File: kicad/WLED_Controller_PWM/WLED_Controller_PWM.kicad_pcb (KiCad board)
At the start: 2 copper layers, 72 x 50 mm, 45 parts, among them J1 USB_C_Receptacle_USB2.0, J2 Conn_01x03, J3 Conn_01x03, J4 Conn_01x03, J6 Conn_01x02, Q1 BC847, Q2 BC847, SW1 SW_RESET, SW2 SW_BOOT, SW3 SW_Push, U1 ESP32-WROOM-32, U2 CH340C, U3 NCP1117-3.3, U4 TSSP58P38, U5 74HC14

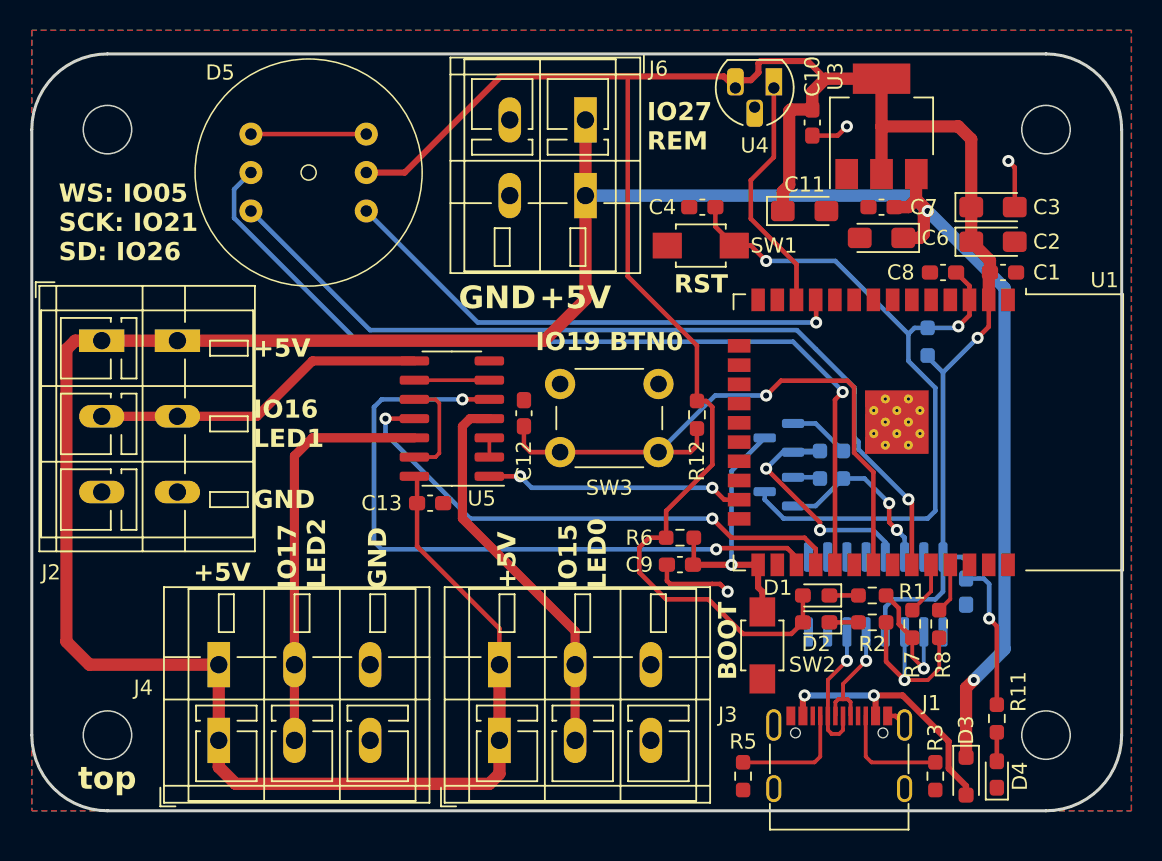
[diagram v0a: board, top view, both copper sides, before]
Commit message: Add PWM Controllers
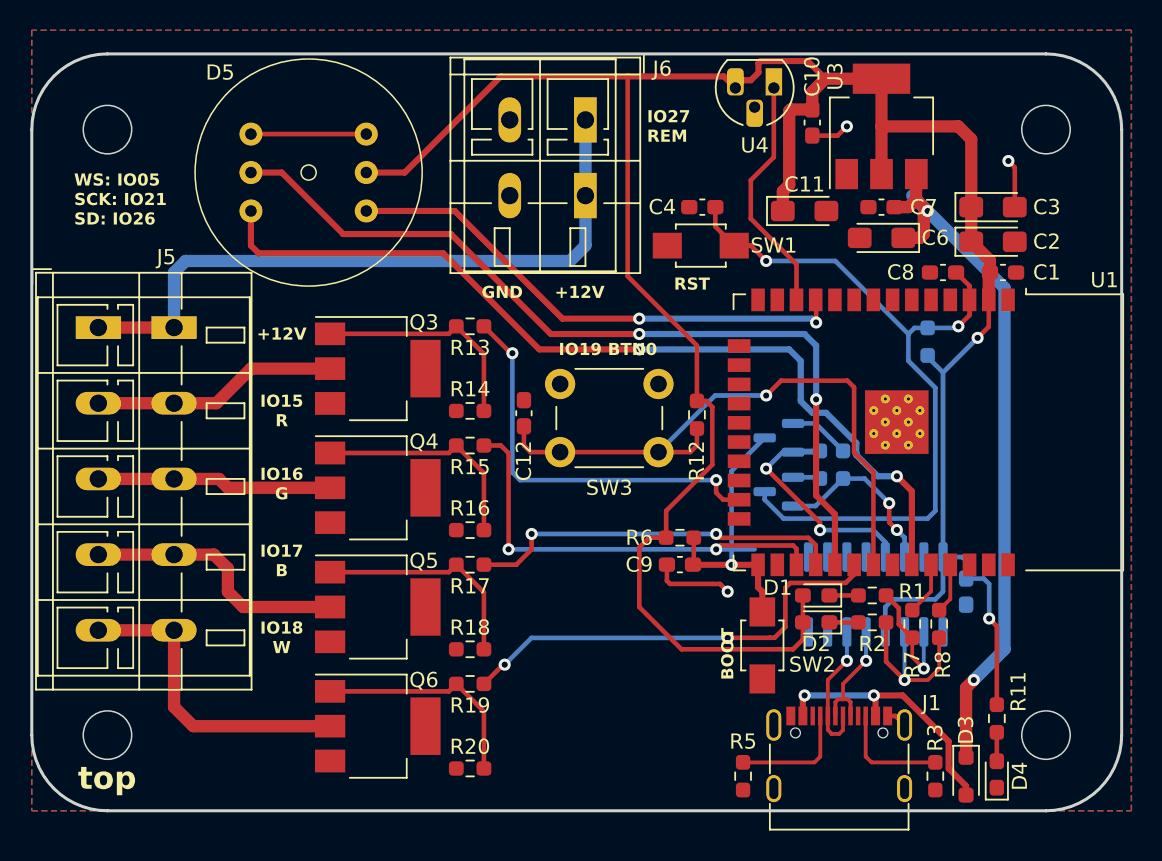
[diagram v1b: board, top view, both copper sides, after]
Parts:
- removed C13: 100n, Capacitor_SMD:C_0603_1608Metric_Pad1.08x0.95mm_HandSolder
- removed J2, J3, J4: Conn_01x03, GioN_Custom:TerminalBlock_WAGO_236-403_1x03_P5.00mm_45Degree
- removed U5: 74HC14, Package_SO:SOIC-14_3.9x8.7mm_P1.27mm
- added J5: Conn_01x05, GioN_Custom:TerminalBlock_WAGO_236-405_1x05_P5.00mm_45Degree, F.Cu at (9.40, -31.9)
- added Q3: IRFL4105PBF, Package_TO_SOT_SMD:SOT-223, F.Cu at (22.9, -29.2)
- added Q4: IRFL4105PBF, Package_TO_SOT_SMD:SOT-223, F.Cu at (22.9, -21.3)
- added Q5: IRFL4105PBF, Package_TO_SOT_SMD:SOT-223, F.Cu at (22.9, -13.5)
- added Q6: IRFL4105PBF, Package_TO_SOT_SMD:SOT-223, F.Cu at (22.9, -5.59)
- added R13: 100R, Resistor_SMD:R_0603_1608Metric_Pad0.98x0.95mm_HandSolder, F.Cu at (29.0, -32.0)
- added R14: 10k, Resistor_SMD:R_0603_1608Metric_Pad0.98x0.95mm_HandSolder, F.Cu at (29.0, -26.4)
- added R15: 100R, Resistor_SMD:R_0603_1608Metric_Pad0.98x0.95mm_HandSolder, F.Cu at (29.0, -24.1)
- added R16: 10k, Resistor_SMD:R_0603_1608Metric_Pad0.98x0.95mm_HandSolder, F.Cu at (29.0, -18.5)
- added R17: 100R, Resistor_SMD:R_0603_1608Metric_Pad0.98x0.95mm_HandSolder, F.Cu at (29.0, -16.3)
- added R18: 10k, Resistor_SMD:R_0603_1608Metric_Pad0.98x0.95mm_HandSolder, F.Cu at (29.0, -10.7)
- added R19: 100R, Resistor_SMD:R_0603_1608Metric_Pad0.98x0.95mm_HandSolder, F.Cu at (29.0, -8.38)
- added R20: 10k, Resistor_SMD:R_0603_1608Metric_Pad0.98x0.95mm_HandSolder, F.Cu at (29.0, -2.79)
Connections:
- J6 pad 1: +5V -> +12V
- U1 pad 23: LED0 -> LED_R
- U1 pad 27: LED1 -> LED_G
- U1 pad 28: LED2 -> LED_B
- U1 pad 30: IO18 -> LED_W
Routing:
- net +5V: track 195.3 -> 48.2 mm
- net LED1: track 45.6 -> 0.00 mm, vias 2 -> 0
- net +12V: track 0.00 -> 44.9 mm
- net LED2: track 35.5 -> 0.00 mm, vias 2 -> 0
- net LED_G: track 0.00 -> 31.0 mm, vias 0 -> 2
- net LED_W: track 0.00 -> 29.6 mm, vias 0 -> 2
- net Net-(J4-Pin_2): track 27.2 -> 0.00 mm
- net LED_R: track 0.00 -> 26.7 mm, vias 0 -> 2
- net Net-(J3-Pin_2): track 25.8 -> 0.00 mm
- net LED_B: track 0.00 -> 25.0 mm, vias 0 -> 2
- net Net-(J2-Pin_2): track 22.2 -> 0.00 mm
- net Net-(J5-Pin_5): track 0.00 -> 20.9 mm
- net Net-(J5-Pin_4): track 0.00 -> 17.6 mm
- net LED0: track 17.1 -> 0.00 mm, vias 2 -> 0
- net Net-(J5-Pin_2): track 0.00 -> 16.3 mm
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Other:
- board text added: "+12V"
- board text added: "IO15 R"
- board text added: "IO16 G"
- board text added: "IO17 B"
- board text added: "IO18 W"
- board text added: "WLED Controller PWM V1 03/2024 Gioulekas Nikos"
- board text removed: "+5V"
- board text removed: "IO15 LED0"
- board text removed: "IO16 LED1"
- board text removed: "IO17 LED2"
- board text removed: "WLED Controller V1 02/2024 Gioulekas Nikos"
